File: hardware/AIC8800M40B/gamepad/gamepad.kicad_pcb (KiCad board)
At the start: 2 copper layers, 195.1 x 88.9 mm, 59 parts, among them J1 Rumble_TL, J10 Micro_SD_Card_Det1, J11 Conn_01x07, J12 Conn_01x10, J13 Conn_01x10, J14 Conn_01x13, J2 Rumble_ML, J3 Rumble_TR, J4 Rumble_MR, J7 Conn_01x03, J8 Conn_01x03, J9 Conn_02x15_Odd_Even, Q1 AO3402, Q2 AO3402, Q3 AO3402, Q4 AO3402, Q5 AO3402, SW1 SW_Push, SW10 SW_Push, SW11 SW_Push, SW12 SW_Push, SW13 SW_Push, SW14 SW_Push, SW15 SW_Push, SW2 SW_Push, SW3 SW_Push, SW4 SW_Push, SW5 SW_Push, SW6 SW_Push, SW7 SW_Push, SW8 SW_Push, SW9 SW_Push, U1 PY32F002AF15P, U2 74HC165, U3 74HC165

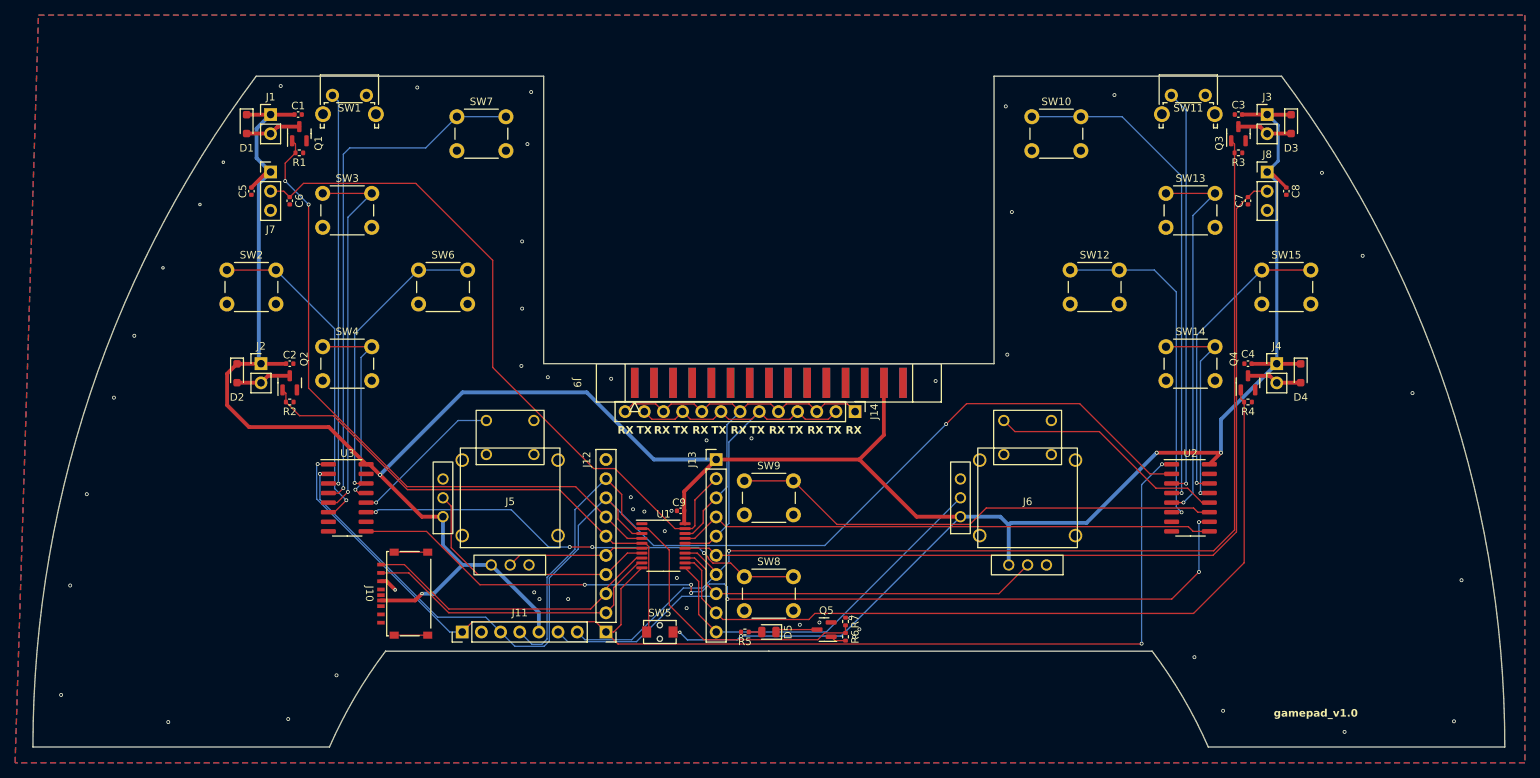
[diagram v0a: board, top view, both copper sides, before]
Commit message: [hardware/aic8800m40b] update gamepad extension board
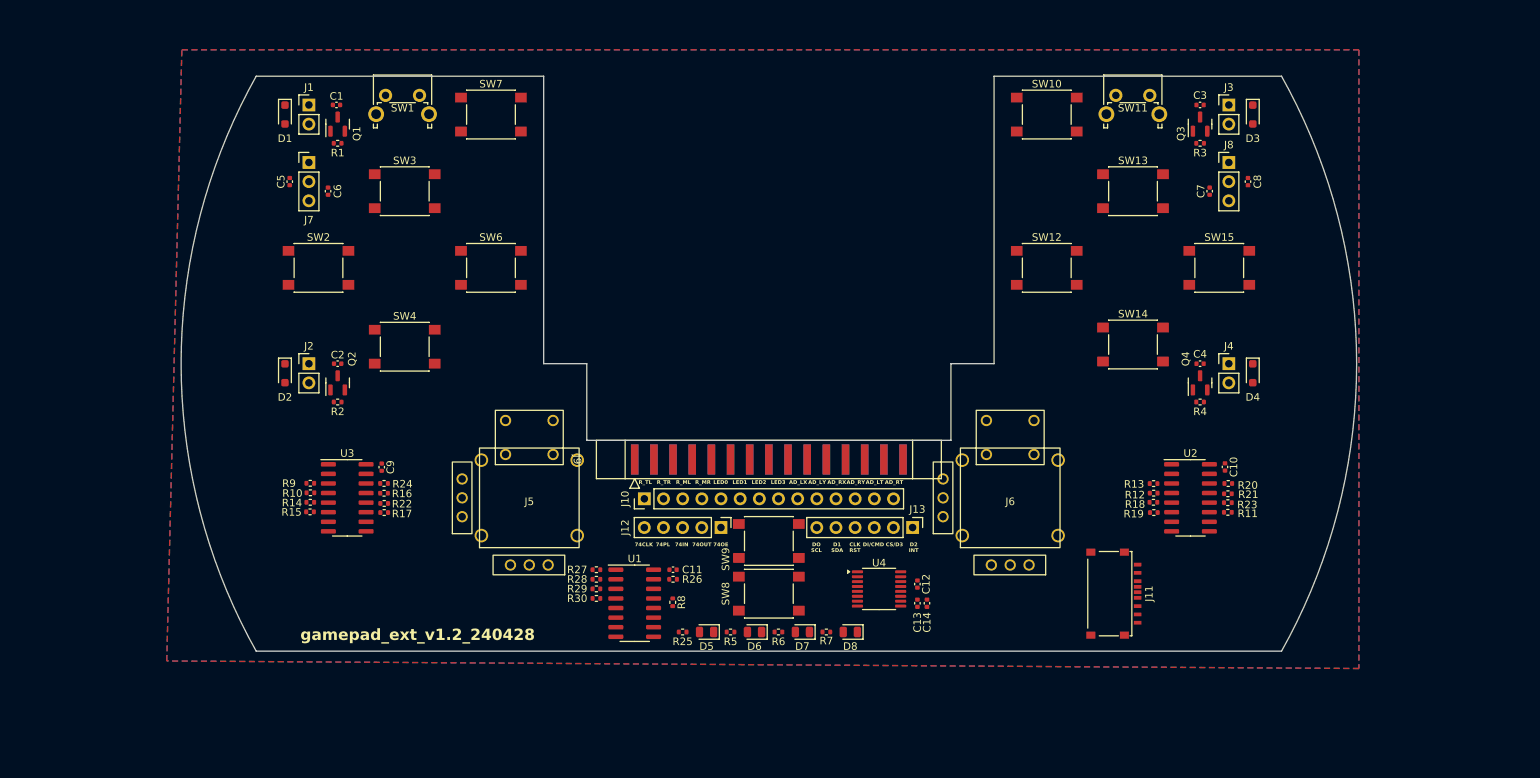
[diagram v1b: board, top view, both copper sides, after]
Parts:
- removed J14: Conn_01x13, Connector_PinHeader_2.54mm:PinHeader_1x13_P2.54mm_Vertical
- removed Q5: AO3402, Package_TO_SOT_SMD:SOT-23
- removed SW5: SW_Push, LC:Key_2Pin_2.9X4.3
- added C10: 100nF, Capacitor_SMD:C_0402_1005Metric, F.Cu at (238.3, 115.3)
- added C11: 100nF, Capacitor_SMD:C_0402_1005Metric, F.Cu at (165.1, 128.9)
- added C12: 100nF, Capacitor_SMD:C_0402_1005Metric, F.Cu at (197.5, 130.8)
- added C13: 1uF, Capacitor_SMD:C_0402_1005Metric, F.Cu at (197.5, 133.3)
- added C14: 100nF, Capacitor_SMD:C_0402_1005Metric, F.Cu at (198.8, 133.3)
- added D6: LED, LED_SMD:LED_0805_2012Metric, F.Cu at (175.9, 137.2)
- added D7: LED, LED_SMD:LED_0805_2012Metric, F.Cu at (182.2, 137.2)
- added D8: LED, LED_SMD:LED_0805_2012Metric, F.Cu at (188.6, 137.2)
- added R10: 4.7K, Resistor_SMD:R_0402_1005Metric, F.Cu at (117.0, 118.7)
- added R11: 4.7K, Resistor_SMD:R_0402_1005Metric, F.Cu at (238.6, 121.3)
- added R12: 4.7K, Resistor_SMD:R_0402_1005Metric, F.Cu at (228.8, 118.8)
- added R13: 4.7K, Resistor_SMD:R_0402_1005Metric, F.Cu at (228.8, 117.5)
- added R14: 4.7K, Resistor_SMD:R_0402_1005Metric, F.Cu at (117.0, 120.0)
- added R15: 4.7K, Resistor_SMD:R_0402_1005Metric, F.Cu at (117.0, 121.2)
- added R16: 4.7K, Resistor_SMD:R_0402_1005Metric, F.Cu at (126.8, 118.8)
- added R17: 4.7K, Resistor_SMD:R_0402_1005Metric, F.Cu at (126.8, 121.3)
- added R18: 4.7K, Resistor_SMD:R_0402_1005Metric, F.Cu at (228.8, 120.0)
- added R19: 4.7K, Resistor_SMD:R_0402_1005Metric, F.Cu at (228.8, 121.3)
- added R20: 4.7K, Resistor_SMD:R_0402_1005Metric, F.Cu at (238.7, 117.5)
- added R21: 4.7K, Resistor_SMD:R_0402_1005Metric, F.Cu at (238.6, 118.8)
- added R22: 4.7K, Resistor_SMD:R_0402_1005Metric, F.Cu at (126.8, 120.1)
- added R23: 4.7K, Resistor_SMD:R_0402_1005Metric, F.Cu at (238.6, 120.0)
- added R24: 4.7K, Resistor_SMD:R_0402_1005Metric, F.Cu at (126.8, 117.5)
- added R25: 100, Resistor_SMD:R_0402_1005Metric, F.Cu at (166.4, 137.2)
- added R26: 0, Resistor_SMD:R_0402_1005Metric, F.Cu at (165.1, 130.2)
- added R27: 0, Resistor_SMD:R_0402_1005Metric, F.Cu at (154.9, 128.9)
- added R28: 0, Resistor_SMD:R_0402_1005Metric, F.Cu at (154.9, 130.2)
- added R29: 0, Resistor_SMD:R_0402_1005Metric, F.Cu at (154.9, 131.4)
- added R30: 0, Resistor_SMD:R_0402_1005Metric, F.Cu at (154.9, 132.7)
- added R8: 4.7K, Resistor_SMD:R_0402_1005Metric, F.Cu at (165.1, 133.2)
- added R9: 4.7K, Resistor_SMD:R_0402_1005Metric, F.Cu at (117.0, 117.5)
- added U4: ADS7830, Package_SO:TSSOP-16_4.4x5mm_P0.65mm, F.Cu at (192.4, 131.5)
- C9: value 1uF -> 100nF
- J10: value Micro_SD_Card_Det1 -> Conn_01x14; footprint VSF:MicroSD_Tiny -> Connector_PinHeader_2.54mm:PinHeader_1x14_P2.54mm_Vertical
- J11: value Conn_01x07 -> Micro_SD_Card_Det1; footprint Connector_PinHeader_2.54mm:PinHeader_1x07_P2.54mm_Vertical -> VSF:MicroSD_Tiny
- J12: value Conn_01x10 -> Conn_01x05; footprint Connector_PinHeader_2.54mm:PinHeader_1x10_P2.54mm_Vertical -> Connector_PinHeader_2.54mm:PinHeader_1x05_P2.54mm_Vertical
- J13: value Conn_01x10 -> Conn_01x06; footprint Connector_PinHeader_2.54mm:PinHeader_1x10_P2.54mm_Vertical -> Connector_PinHeader_2.54mm:PinHeader_1x06_P2.54mm_Vertical
- R6: value 1.5k -> 100
- R7: value 100k -> 100
- SW10, SW12, SW13, SW14, SW15, SW2, SW3, SW4, SW6, SW7, SW8, SW9: footprint Button_Switch_THT:SW_PUSH_6mm -> Button_Switch_SMD:SW_Push_1P1T_NO_6x6mm_H9.5mm
- U1: value PY32F002AF15P -> 74HC595; footprint Package_SO:TSSOP-20_4.4x6.5mm_P0.65mm -> Package_SO:SOP-16_3.9x9.9mm_P1.27mm
- moved J11 89.7 mm to (226.7, 132.1)
- moved C9 40.0 mm to (126.5, 115.3), turned to -90 degrees
- moved J10 37.1 mm to (161.3, 119.5), turned to 90 degrees
- moved J13 27.6 mm to (196.8, 123.3), turned to -90 degrees
- moved J12 20.6 mm to (171.4, 123.3), turned to -90 degrees
- moved SW2 12.1 mm to (118.1, 88.9)
- moved SW3 10.9 mm to (129.5, 78.7)
- moved SW4 10.9 mm to (129.5, 99.3)
- moved J9 10.2 mm to (177.8, 114.3)
- moved SW6 9.60 mm to (141.0, 88.9)
- moved R6 8.91 mm to (179.1, 137.2), turned to 0 degrees
- moved SW9 8.60 mm to (177.8, 125.1)
- moved U1 8.52 mm to (160.0, 133.3)
- moved D5 8.26 mm to (169.5, 137.2)
- moved SW11 7.35 mm to (223.8, 66.0)
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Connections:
- net /_USB_DM renamed /USB_DM
- net /_USB_DP renamed /USB_DP
- C1 pad 1: /VCC -> /5V
- C2 pad 1: /VCC -> /5V
- C3 pad 1: /VCC -> /5V
- C4 pad 1: /VCC -> /5V
- D1 pad 1: /VCC -> /5V
- D2 pad 1: /VCC -> /5V
- D3 pad 1: /VCC -> /5V
- D4 pad 1: /VCC -> /5V
- D5 pad 1: /LED- -> GND
- D5 pad 2: /LED+ -> Net-(D5-A)
- J1 pad 1: /VCC -> /5V
- J10 pad 1: unconnected-(J10-DAT2-Pad1) -> /RUMBLE_TL
- J10 pad 10: GND -> /AD_LY
- J10 pad 2: unconnected-(J10-DAT3/CD-Pad2) -> /RUMBLE_TR
- J10 pad 3: unconnected-(J10-CMD-Pad3) -> /RUMBLE_ML
- J10 pad 4: /VCC -> /RUMBLE_MR
- J10 pad 5: unconnected-(J10-CLK-Pad5) -> /LED0
- J10 pad 6: GND -> /LED1
- J10 pad 7: /IIC_SCL -> /LED2
- J10 pad 8: /IIC_SDA -> /LED3
- J10 pad 9: unconnected-(J10-DET-Pad9) -> /AD_LX
- J11 pad 1: /74PL -> /INT
- J11 pad 2: GND -> /CS
- J11 pad 3: /74CLK -> /DI
- J11 pad 4: /LED -> /VCC
- J11 pad 5: /VCC -> /CLK
- J11 pad 6: /AD_RX -> GND
- J11 pad 7: /RUMBLE_TR -> /DO
- J12 pad 1: /74PL -> /74OE
- J12 pad 2: /IIC_SCL -> /74OUT
- J12 pad 3: /IIC_SDA -> /74IN
- J12 pad 4: /AD_LY -> /74PL
- J12 pad 5: /AD_LX -> /74CLK
- J13 pad 1: /VCC -> /INT
- J13 pad 2: /AD_LT -> /CS
- J13 pad 3: /UART_RX -> /DI
- J13 pad 4: /74IN -> /CLK
- J13 pad 5: /UART_TX -> /SDA
- J13 pad 6: /AD_RT -> /DO
- J2 pad 1: /VCC -> /5V
- J3 pad 1: /VCC -> /5V
- J4 pad 1: /VCC -> /5V
- J5 pad 4: /VCC -> GND
- J5 pad 6: GND -> /VCC
- J6 pad 4: /VCC -> GND
- J6 pad 6: GND -> /VCC
- J9 pad 29: /USB5V_OUT -> /5V
- R5 pad 1: /VCC -> /LED1
- R5 pad 2: /LED+ -> Net-(D6-A)
- R6 pad 1: Net-(Q5-G) -> /LED2
- R6 pad 2: /LED -> Net-(D7-A)
- R7 pad 1: GND -> /LED3
- R7 pad 2: /LED -> Net-(D8-A)
- U1 pad 1: GND -> Net-(U1-QB)
- U1 pad 10: /74PL -> /VCC
- U1 pad 11: /AD_RY -> /74CLK
- U1 pad 12: /RUMBLE_MR -> /74PL
- U1 pad 13: /AD_RX -> /74OE
- U1 pad 14: /RUMBLE_TR -> /74OUT
- U1 pad 15: /AD_RT -> Net-(U1-QA)
- U1 pad 16: /UART_TX -> /VCC
- U1 pad 2: /LED -> Net-(U1-QC)
- U1 pad 3: /74CLK -> Net-(U1-QD)
- U1 pad 4: /RUMBLE_TL -> Net-(U1-QE)
- U1 pad 5: /RUMBLE_ML -> /LED1
- U1 pad 6: /AD_LX -> /LED2
- U1 pad 7: /AD_LY -> /LED3
- U1 pad 8: /IIC_SDA -> GND
- U1 pad 9: /IIC_SCL -> unconnected-(U1-QH'-Pad9)
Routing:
- net /VCC: track 396.3 -> 0.00 mm, vias 6 -> 0
- net /74CLK: track 162.0 -> 0.00 mm, vias 2 -> 0
- net /74PL: track 161.8 -> 0.00 mm, vias 3 -> 0
- net /RUMBLE_TR: track 151.7 -> 0.00 mm, vias 1 -> 0
- net Net-(U2-DS): track 126.2 -> 0.00 mm, vias 6 -> 0
- net /AD_RT: track 122.6 -> 0.00 mm
- net /RUMBLE_MR: track 105.6 -> 0.00 mm
- net /AD_LT: track 92.2 -> 0.00 mm
- net /RUMBLE_TL: track 87.2 -> 0.00 mm, vias 2 -> 0
- net /LED: track 76.9 -> 0.00 mm
- net /AD_RX: track 74.1 -> 0.00 mm
- net /74IN: track 71.5 -> 0.00 mm
- net /SW_ML: track 70.1 -> 0.00 mm, vias 1 -> 0
- net /RUMBLE_ML: track 69.3 -> 0.00 mm
- net /SW_MR: track 66.4 -> 0.00 mm, vias 1 -> 0
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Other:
- board size 195.1 x 88.9 mm -> 155.8 x 76.2 mm
- board text added: "74CLK"
- board text added: "74IN"
- board text added: "74OE"
- board text added: "74OUT"
- board text added: "74PL"
- board text added: "AD_LT"
- board text added: "AD_LX"
- board text added: "AD_LY"
- board text added: "AD_RT"
- board text added: "AD_RX"
- board text added: "AD_RY"
- board text added: "CLK"
- board text added: "CS/D3"
- board text added: "D1"
- board text added: "D2"
- board text added: "DI/CMD"
- board text added: "DO"
- board text added: "INT"
- board text added: "LED0"
- board text added: "LED1"
- board text added: "LED2"
- board text added: "LED3"
- board text added: "RST"
- board text added: "R_ML"
- board text added: "R_MR"
- board text added: "R_TL"
- board text added: "R_TR"
- board text added: "SCL"
- board text added: "SDA"
- board text added: "gamepad_ext_v1.2_240428"
- board text removed: "RX"
- board text removed: "TX"
- board text removed: "gamepad_v1.0"
